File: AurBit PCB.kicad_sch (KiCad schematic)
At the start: 1 part

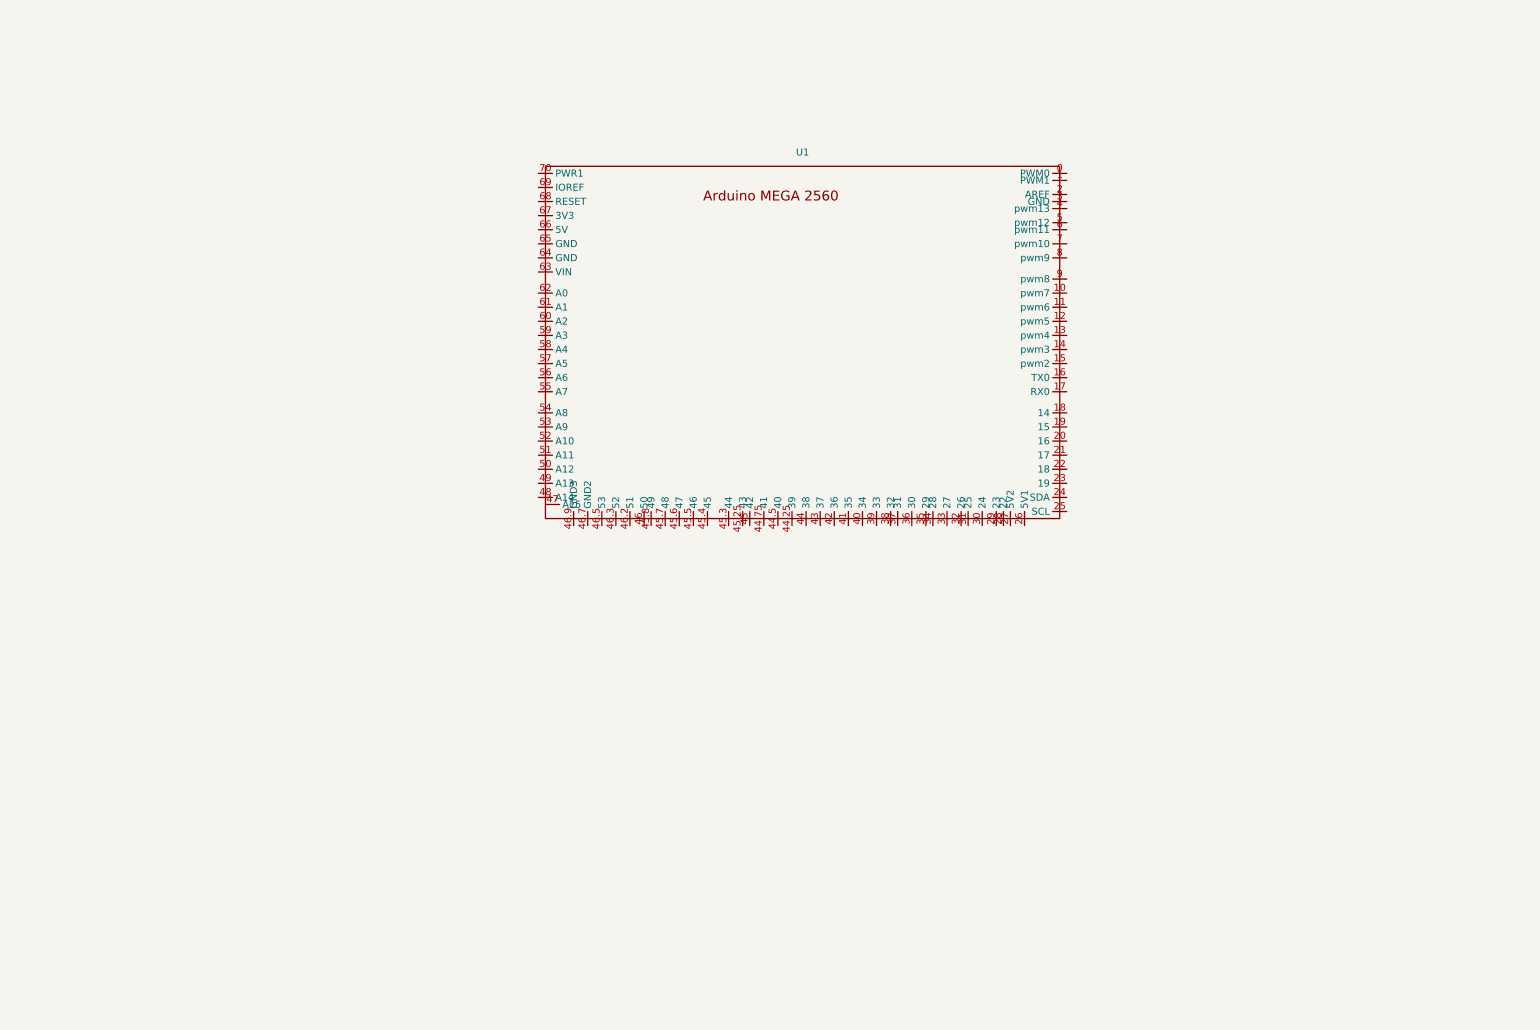
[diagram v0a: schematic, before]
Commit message: Save AurBit KiCad schematic and custom symbols
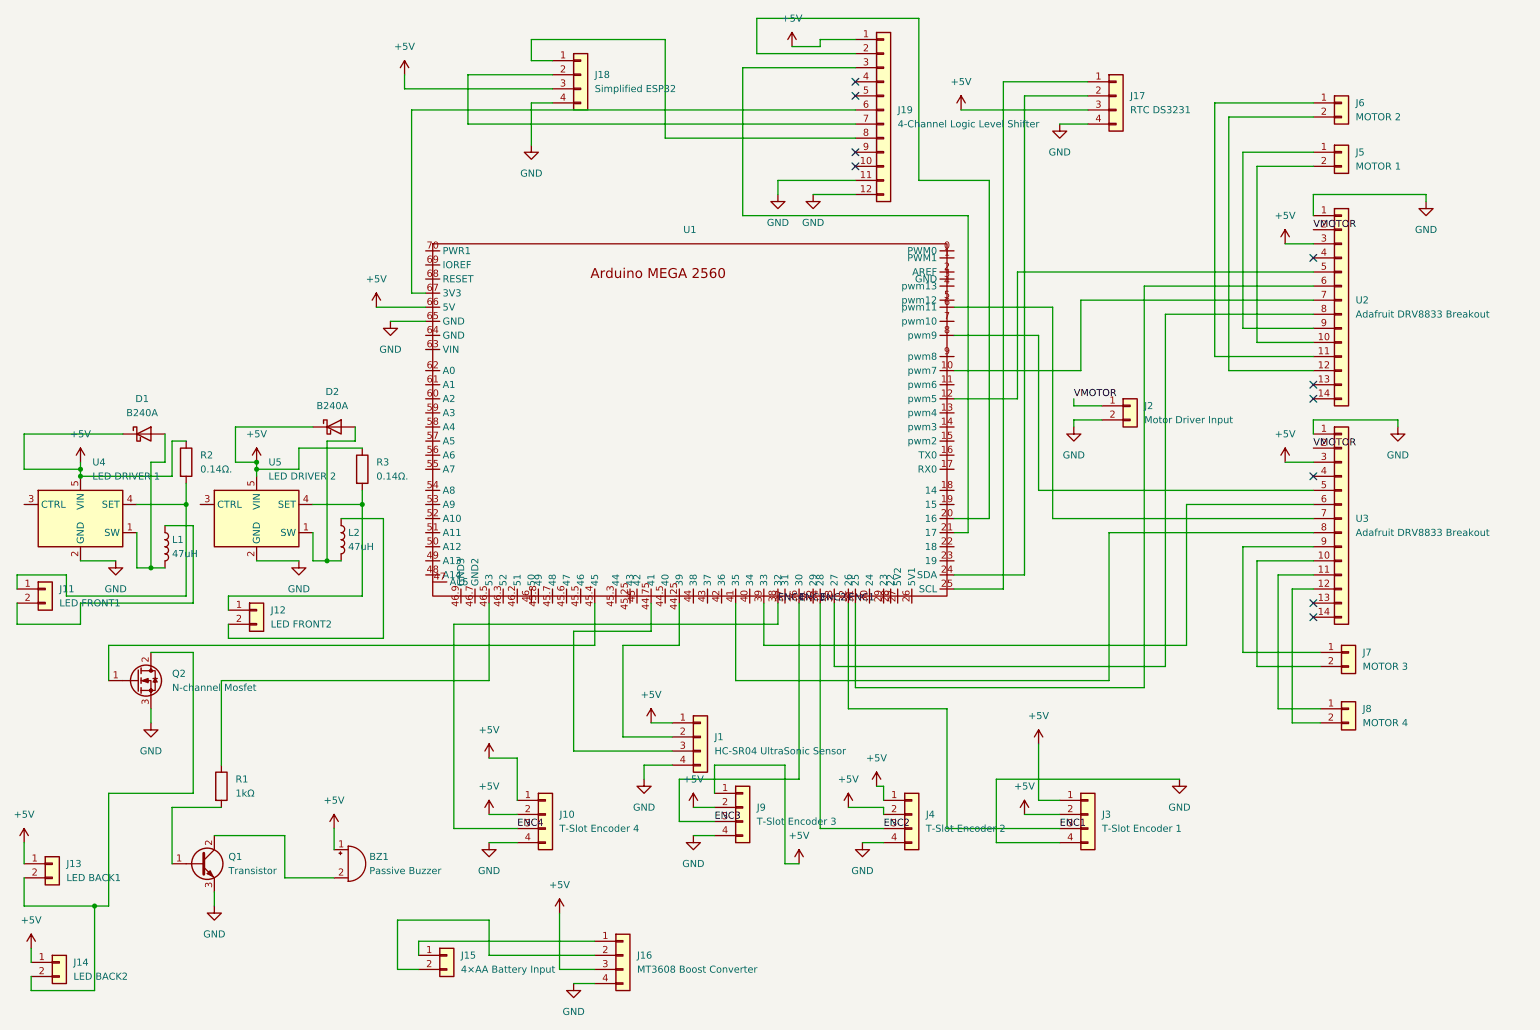
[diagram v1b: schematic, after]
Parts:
- added BZ1: Passive Buzzer, symbol Device:Buzzer
- added D1, D2: B240A, symbol Device:D_Schottky
- added J1: HC-SR04 UltraSonic Sensor, symbol Connector_Generic:Conn_01x04
- added J10: T-Slot Encoder 4, symbol Connector_Generic:Conn_01x04
- added J11: LED FRONT1, symbol Connector_Generic:Conn_01x02
- added J12: LED FRONT2, symbol Connector_Generic:Conn_01x02
- added J13: LED BACK1, symbol Connector_Generic:Conn_01x02
- added J14: LED BACK2, symbol Connector_Generic:Conn_01x02
- added J15: 4×AA Battery Input, symbol Connector_Generic:Conn_01x02
- added J16: MT3608 Boost Converter, symbol Connector_Generic:Conn_01x04
- added J17: RTC DS3231, Package_TO_SOT_SMD:TO-263-7_TabPin8, symbol Connector_Generic:Conn_01x04
- added J18: Simplified ESP32, Package_TO_SOT_SMD:TO-263-7_TabPin8, symbol Connector_Generic:Conn_01x04
- added J19: 4-Channel Logic Level Shifter, symbol Connector_Generic:Conn_01x12
- added J2: Motor Driver Input, symbol Connector_Generic:Conn_01x02
- added J3: T-Slot Encoder 1, symbol Connector_Generic:Conn_01x04
- added J4: T-Slot Encoder 2, symbol Connector_Generic:Conn_01x04
- added J5: MOTOR 1, symbol Connector_Generic:Conn_01x02
- added J6: MOTOR 2, symbol Connector_Generic:Conn_01x02
- added J7: MOTOR 3, symbol Connector_Generic:Conn_01x02
- added J8: MOTOR 4, symbol Connector_Generic:Conn_01x02
- added J9: T-Slot Encoder 3, symbol Connector_Generic:Conn_01x04
- added L1, L2: 47uH, symbol Device:L
- added Q1: Transistor, symbol Transistor_BJT:Q_NPN_BCE
- added Q2: N-channel Mosfet, symbol Transistor_FET:Q_NMOS_GDS
- added R1: 1kΩ, symbol Device:R
- added R2, R3: 0.14Ω., symbol Device:R
- added U2: Adafruit DRV8833 Breakout, Connector_PinSocket_2.54mm:PinSocket_2x07_P2.54mm_Vertical_SMD, symbol Connector_Generic:Conn_01x14
- added U3: Adafruit DRV8833 Breakout, symbol Adafruit_DRV8833_Breakout:Adafruit_DRV8833_Breakout
- added U4: LED DRIVER 1, Package_TO_SOT_SMD:TSOT-23-5, symbol Driver_LED:AL8860WT
- added U5: LED DRIVER 2, Package_TO_SOT_SMD:TSOT-23-5, symbol Driver_LED:AL8860WT
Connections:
- net at U1.10 (pwm7): now also U2.7 (BIN1)
- net at U1.12 (pwm5): now also U2.5 (AIN1)
- net at U1.20 (16): now also J19.2 (HV1)
- net at U1.21 (17): now also J19.3 (HV2)
- net at U1.24 (SDA): now also J17.2 (SDA)
- net at U1.25 (SCL): now also J17.1 (SCL)
- net at U1.31 (25): now also U2.6 (AIN2)
- net ENC1: now reaches U1.32 (26)
- net ENC1: now also J3.3 (OUT)
- net at U1.33 (27): now also U2.8 (BIN2)
- net ENC2: now reaches U1.34 (28)
- net ENC2: now also J4.3 (OUT)
- net ENC3: now reaches U1.36 (30)
- net ENC3: now also J9.3 (OUT)
- net ENC4: now reaches U1.38 (32)
- net ENC4: now also J10.3 (OUT)
- net at U1.39 (33): now also U3.6 (AIN2)
- net at U1.41 (35): now also U3.8 (BIN2)
- net at U1.44.25 (39): now also J1.2 (TRIG)
- net at U1.44.75 (41): now also J1.3 (ECHO)
- net at U1.45.4 (45): now also Q2.1 (G)
- net at U1.46.5 (53): now also R1.1
- net at U1.6 (pwm11): now also U3.7 (BIN1)
- net GND: now reaches U1.65 (GND)
- net GND: now also J1.4 (GND), J10.4 (-), J16.4 (VOUT-), J17.4 (GND), J18.4 (VBUS(5V)), J19.11 (GND), J19.12 (GND), J2.2 (GND), J3.4 (-), J4.4 (-), J9.4 (-), Q1.3 (E), Q2.3 (S), U2.1 (GND), U3.1 (GND), U4.2 (GND), U5.2 (GND)
- net +5V: now reaches U1.66 (5V)
- net +5V: now also BZ1.1 (+), D1.1 (K), D2.1 (K), J1.1 (VCC), J10.1 (+), J10.2 (L), J13.1 (+), J14.1 (+), J16.3 (VOUT+), J17.3 (VCC), J18.3 (GND), J19.1 (HV), J3.1 (+), J3.2 (L), J4.1 (+), J4.2 (L), J9.1 (+), J9.2 (L), R2.1, R3.1, U2.3 (SLP), U3.3 (SLP), U4.5 (VIN), U5.5 (VIN)
- net at U1.67 (3V3): now also J19.6 (LV)
- net at U1.8 (pwm9): now also U3.5 (AIN1)
- new net: D1.2 (A), L1.2 (-), U4.1 (SW)
- new net: J11.1 (+), R2.2, U4.4 (SET)
- new net: J18.2 (RX0), J19.7 (LV1)
- new net: J18.1 (TXO), J19.8 (LV2)
- new net: J7.2 (Pin_2), U3.10 (AOUT2)
- new net: J8.1 (Pin_1), U3.11 (BOUT1)
- new net: J8.2 (Pin_2), U3.12 (BOUT2)
- new net: J7.1 (Pin_1), U3.9 (AOUT1)
- new net: J11.2 (-), L1.1 (+)
- new net: J12.2 (-), L2.1 (+)
- new net: D2.2 (A), L2.2 (-), U5.1 (SW)
- new net: J5.1 (Pin_1), U2.9 (AOUT1)
- new net: J5.2 (Pin_2), U2.10 (AOUT2)
- new net: J15.1 (+), J16.1 (VIN+)
- new net: J15.2 (-), J16.2 (VIN-)
- new net: Q1.1 (B), R1.2
- new net: BZ1.2 (-), Q1.2 (C)
- new net: J6.1 (Pin_1), U2.11 (BOUT1)
- new net: J6.2 (Pin_2), U2.12 (BOUT2)
- new net: J13.2 (-), J14.2 (-), Q2.2 (D)
- new net: J12.1 (+), R3.2, U5.4 (SET)
- new net VMOTOR: J2.1 (VMOTOR+), U2.2 (VM), U3.2 (VM)
- no-connect marks 0 -> 10
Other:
- moved on the sheet: U1
